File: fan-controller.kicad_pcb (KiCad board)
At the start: 2 copper layers, 33 x 16 mm, 17 parts, among them J1 PWR, J2 PTC, J3 FAN, J4 Prog, Q1 AO3401A, U1 PY32F002A

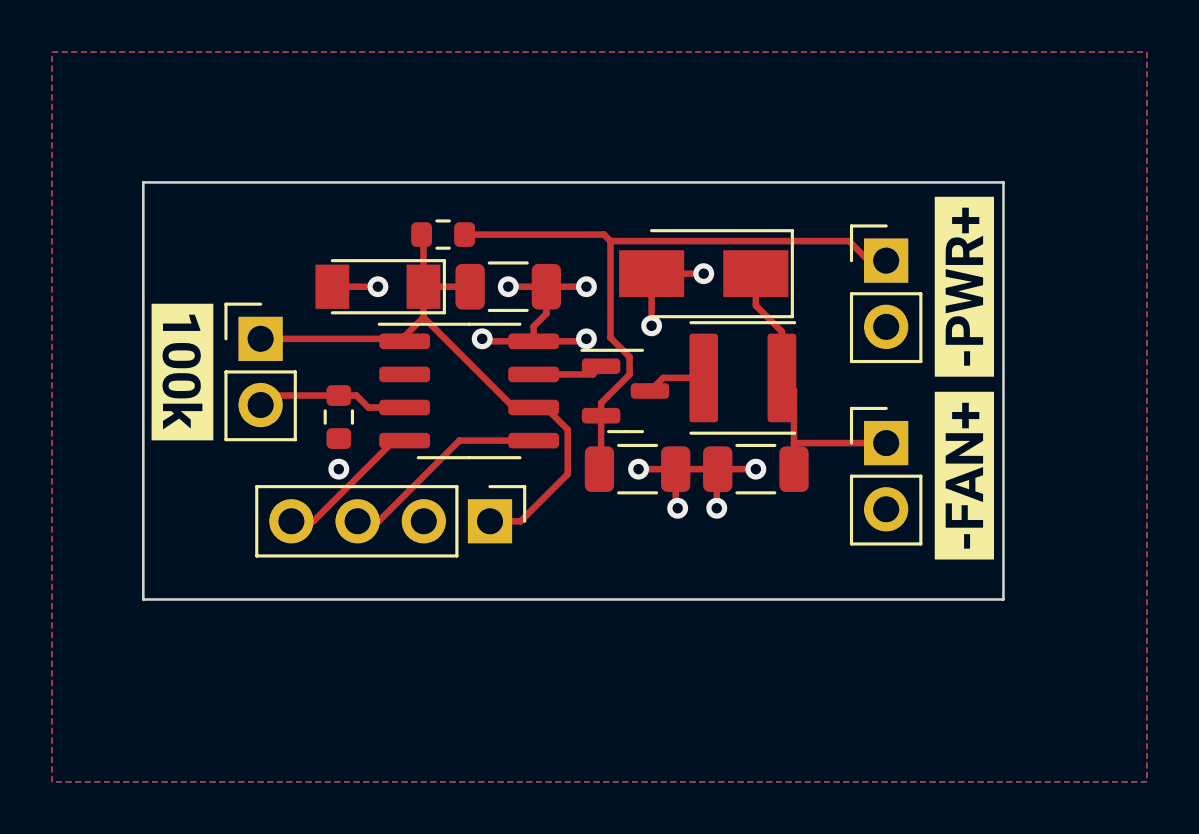
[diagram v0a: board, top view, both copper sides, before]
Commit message: Fix ERC
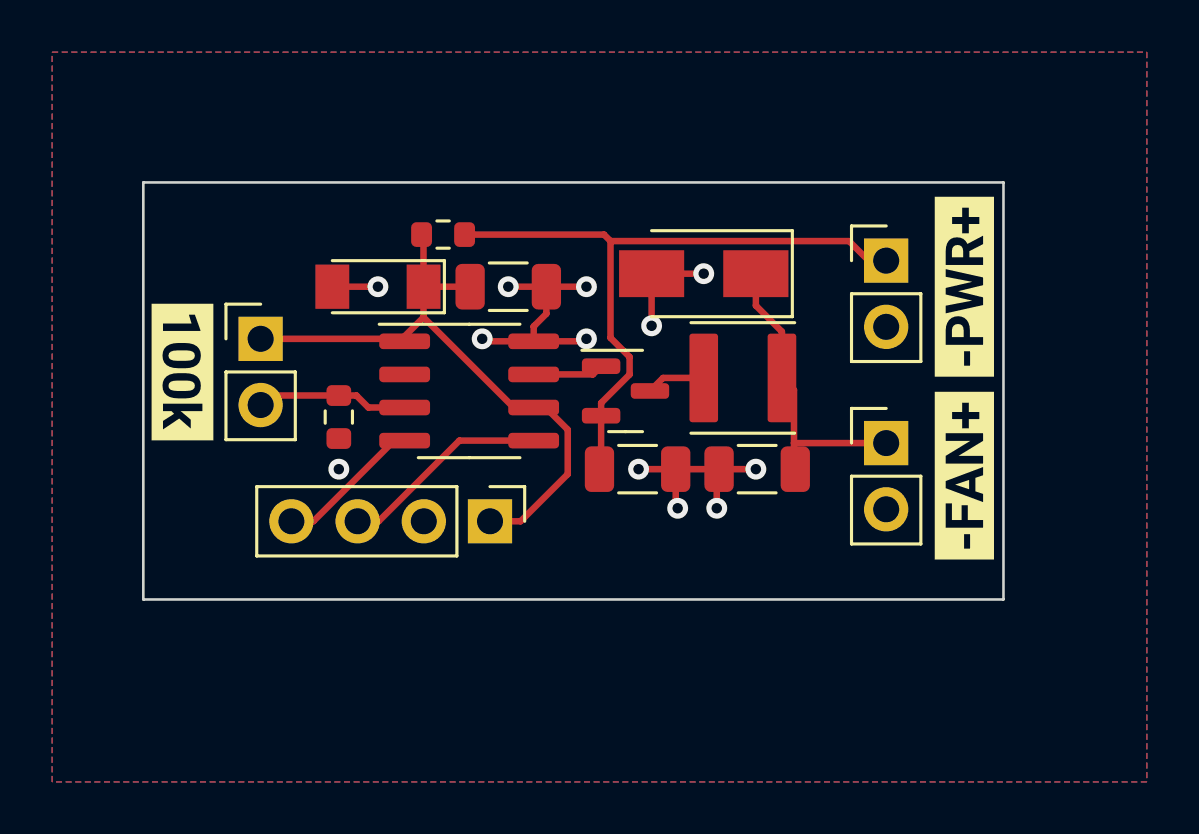
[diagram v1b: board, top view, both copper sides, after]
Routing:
- net +3.3V: track 24.8 -> 23.4 mm
- net VPP: track 26.6 -> 25.4 mm
- net Net-(C3-Pad1): track 12.1 -> 11.0 mm
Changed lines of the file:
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@@
     (tags "inductor abracon smd shielded")
     (property "LCSC" "C38117")
-    (property "Sheetfile" "/home/user/dev/hardware/fan-controller/fan-controller.sch")
+    (property "Sheetfile" "fan-controller.kicad_sch")
     (property "Sheetname" "")
     (attr smd)
@@
     (tags "resistor")
     (property "LCSC" "C25803")
-    (property "Sheetfile" "/home/user/dev/hardware/fan-controller/fan-controller.sch")
+    (property "Sheetfile" "fan-controller.kicad_sch")
     (property "Sheetname" "")
     (attr smd)
@@
     (property "Description" "50V+")
     (property "LCSC" "C13585")
-    (property "Sheetfile" "/home/user/dev/hardware/fan-controller/fan-controller.sch")
+    (property "Sheetfile" "fan-controller.kicad_sch")
     (property "Sheetname" "")
     (attr smd)
@@
   )
   (footprint "Resistor_SMD:R_1206_3216Metric" (layer "F.Cu")
-    (at 122 63 180)
+    (at 122.05 63 180)
     (descr "Resistor SMD 1206 (3216 Metric), square (rectangular) end terminal, IPC_7351 nominal, (Body size source: IPC-SM-782 page 72, https://www.pcb-3d.com/wordpress/wp-content/uploads/ipc-sm-782a_amendment_1_and_2.pdf), generated with kicad-footprint-generator")
     (tags "resistor")
     (property "Description" "50V+")
     (property "LCSC" "C13585")
-    (property "Sheetfile" "/home/user/dev/hardware/fan-controller/fan-controller.sch")
+    (property "Sheetfile" "fan-controller.kicad_sch")
     (property "Sheetname" "")
     (attr smd)
@@
     (descr "Through hole straight pin header, 1x02, 2.54mm pitch, single row")
     (tags "Through hole pin header THT 1x02 2.54mm single row")
-    (property "Sheetfile" "/home/user/dev/hardware/fan-controller/fan-controller.sch")
+    (property "Sheetfile" "fan-controller.kicad_sch")
     (property "Sheetname" "")
     (attr through_hole)
@@
     (descr "Through hole straight pin header, 1x02, 2.54mm pitch, single row")
     (tags "Through hole pin header THT 1x02 2.54mm single row")
-    (property "Sheetfile" "/home/user/dev/hardware/fan-controller/fan-controller.sch")
+    (property "Sheetfile" "fan-controller.kicad_sch")
     (property "Sheetname" "")
     (attr through_hole)
@@
     (tags "Diode Mini-MELF (SOD-80)")
     (property "LCSC" "C8056")
-    (property "Sheetfile" "/home/user/dev/hardware/fan-controller/fan-controller.sch")
+    (property "Sheetfile" "fan-controller.kicad_sch")
     (property "Sheetname" "")
     (attr smd)
@@
     (descr "Through hole straight pin header, 1x04, 2.54mm pitch, single row")
     (tags "Through hole pin header THT 1x04 2.54mm single row")
-    (property "Sheetfile" "/home/user/dev/hardware/fan-controller/fan-controller.sch")
+    (property "Sheetfile" "fan-controller.kicad_sch")
     (property "Sheetname" "")
     (attr through_hole)
@@
     (attr board_only exclude_from_pos_files exclude_from_bom)
     (fp_text reference "kibuzzard-63E17401" (at 0 -4.233917 90) (layer "F.SilkS") hide
-      (effects (font (size 0 0)))
+      (effects (font (size 0 0) (thickness 0.15)))
     )
     (fp_text value "G***" (at 0 4.233917 90) (layer "F.SilkS") hide
-      (effects (font (size 0 0)))
+      (effects (font (size 0 0) (thickness 0.15)))
     )
     (fp_poly (pts
@@
     (tags "resistor")
     (property "LCSC" "C25804")
-    (property "Sheetfile" "/home/user/dev/hardware/fan-controller/fan-controller.sch")
+    (property "Sheetfile" "fan-controller.kicad_sch")
     (property "Sheetname" "")
     (attr smd)
@@
     (attr board_only exclude_from_pos_files exclude_from_bom)
     (fp_text reference "kibuzzard-63E173EF" (at 0 -4.184695 90) (layer "F.SilkS") hide
-      (effects (font (size 0 0)))
+      (effects (font (size 0 0) (thickness 0.15)))
     )
     (fp_text value "G***" (at 0 4.184695 90) (layer "F.SilkS") hide
-      (effects (font (size 0 0)))
+      (effects (font (size 0 0) (thickness 0.15)))
     )
     (fp_poly (pts
@@
     (property "Description" "50V+")
     (property "LCSC" "C13585")
-    (property "Sheetfile" "/home/user/dev/hardware/fan-controller/fan-controller.sch")
+    (property "Sheetfile" "fan-controller.kicad_sch")
     (property "Sheetname" "")
     (attr smd)
@@
     (tags "Diode SMA (DO-214AC)")
     (property "LCSC" "C2480")
-    (property "Sheetfile" "/home/user/dev/hardware/fan-controller/fan-controller.sch")
+    (property "Sheetfile" "fan-controller.kicad_sch")
     (property "Sheetname" "")
     (attr smd)
@@
     (attr board_only exclude_from_pos_files exclude_from_bom)
     (fp_text reference "kibuzzard-63E173E4" (at 0 -4.184695 90) (layer "F.SilkS") hide
-      (effects (font (size 0 0)))
+      (effects (font (size 0 0) (thickness 0.15)))
     )
     (fp_text value "G***" (at 0 4.184695 90) (layer "F.SilkS") hide
-      (effects (font (size 0 0)))
+      (effects (font (size 0 0) (thickness 0.15)))
     )
     (fp_poly (pts
@@
     (tags "SOIC SO")
     (property "LCSC" "C5128435")
-    (property "Sheetfile" "/home/user/dev/hardware/fan-controller/fan-controller.sch")
+    (property "Sheetfile" "fan-controller.kicad_sch")
     (property "Sheetname" "")
     (attr smd)
@@
       (net 1 "+3.3V") (pinfunction "VCC") (pintype "power_in"))
     (pad "2" smd roundrect (at -2.475 -0.635) (size 1.95 0.6) (layers "F.Cu" "F.Paste" "F.Mask") (roundrect_rratio 0.25)
-      (net 10 "unconnected-(U1-Pad2)") (pinfunction "PA4/PA10") (pintype "bidirectional"))
+      (net 10 "unconnected-(U1-Pad2)") (pinfunction "PA4/PA10") (pintype "bidirectional+no_connect"))
     (pad "3" smd roundrect (at -2.475 0.635) (size 1.95 0.6) (layers "F.Cu" "F.Paste" "F.Mask") (roundrect_rratio 0.25)
       (net 5 "/TEMP_SENSE") (pinfunction "PA3") (pintype "bidirectional"))
@@
     (tags "SOT TO_SOT_SMD")
     (property "LCSC" "C15127")
-    (property "Sheetfile" "/home/user/dev/hardware/fan-controller/fan-controller.sch")
+    (property "Sheetfile" "fan-controller.kicad_sch")
     (property "Sheetname" "")
     (attr smd)
@@
     (descr "Through hole straight pin header, 1x02, 2.54mm pitch, single row")
     (tags "Through hole pin header THT 1x02 2.54mm single row")
-    (property "Sheetfile" "/home/user/dev/hardware/fan-controller/fan-controller.sch")
+    (property "Sheetfile" "fan-controller.kicad_sch")
     (property "Sheetname" "")
     (attr through_hole)
@@
   (segment (start 111.8 65) (end 112.9753 65) (width 0.25) (layer "F.Cu") (net 1))
   (segment (start 109.25 57.1753) (end 108.525 57.9003) (width 0.25) (layer "F.Cu") (net 1))
-  (segment (start 109.25 54.075) (end 109.175 54) (width 0.25) (layer "F.Cu") (net 1))
   (segment (start 111.0375 56) (end 109.25 56) (width 0.25) (layer "F.Cu") (net 1))
   (segment (start 109.25 56) (end 109.25 57.1753) (width 0.25) (layer "F.Cu") (net 1))
   (segment (start 112.9753 65) (end 114.783 63.1923) (width 0.25) (layer "F.Cu") (net 1))
-  (segment (start 112.7097 60.635) (end 113.475 60.635) (width 0.25) (layer "F.Cu") (net 1))
   (segment (start 109.25 57.1753) (end 112.7097 60.635) (width 0.25) (layer "F.Cu") (net 1))
-  (segment (start 113.933 60.635) (end 113.475 60.635) (width 0.25) (layer "F.Cu") (net 1))
-  (segment (start 108.525 58) (end 108.525 58.095) (width 0.25) (layer "F.Cu") (net 1))
   (segment (start 108.525 57.9003) (end 108.525 58) (width 0.25) (layer "F.Cu") (net 1))
   (segment (start 114.783 63.1923) (end 114.783 61.485) (width 0.25) (layer "F.Cu") (net 1))
@@
   (segment (start 122 63) (end 121 63) (width 0.25) (layer "F.Cu") (net 2))
   (segment (start 113.9625 56) (end 113.9625 57.0375) (width 0.25) (layer "F.Cu") (net 2))
-  (segment (start 113.9625 56) (end 114 56.0375) (width 0.25) (layer "F.Cu") (net 2))
   (segment (start 115.405 58.095) (end 115.5 58) (width 0.25) (layer "F.Cu") (net 2))
   (segment (start 113.475 58.095) (end 111.595 58.095) (width 0.25) (layer "F.Cu") (net 2))
@@
   (segment (start 116.0625 60.95) (end 116.0625 60.4625) (width 0.25) (layer "F.Cu") (net 3))
   (segment (start 116.4246 57.9644) (end 116.4246 54.25) (width 0.25) (layer "F.Cu") (net 3))
-  (segment (start 116 63) (end 116.0625 62.9375) (width 0.25) (layer "F.Cu") (net 3))
-  (segment (start 127.5 55) (end 126.3247 55) (width 0.25) (layer "F.Cu") (net 3))
   (segment (start 116.0625 62.9375) (end 116.0625 60.95) (width 0.25) (layer "F.Cu") (net 3))
   (segment (start 123 57.7253) (end 122 56.7253) (width 0.25) (layer "F.Cu") (net 4))
-  (segment (start 127.5 62) (end 126.3247 62) (width 0.25) (layer "F.Cu") (net 4))
   (segment (start 123.4625 59.9625) (end 123 59.5) (width 0.25) (layer "F.Cu") (net 4))
   (segment (start 123 59.5) (end 123 57.7253) (width 0.25) (layer "F.Cu") (net 4))
@@
   (segment (start 123.4625 62) (end 126.3247 62) (width 0.25) (layer "F.Cu") (net 4))
   (segment (start 122 55.5) (end 122 56.7253) (width 0.25) (layer "F.Cu") (net 4))
-  (segment (start 106 60.3575) (end 106 60.175) (width 0.25) (layer "F.Cu") (net 5))
   (segment (start 106 60.175) (end 102.825 60.175) (width 0.25) (layer "F.Cu") (net 5))
   (segment (start 108.525 60.635) (end 107.135 60.635) (width 0.25) (layer "F.Cu") (net 5))
@@
   (segment (start 110.6229 61.905) (end 113.475 61.905) (width 0.25) (layer "F.Cu") (net 6))
   (segment (start 107.5279 65) (end 110.6229 61.905) (width 0.25) (layer "F.Cu") (net 6))
-  (segment (start 108.1209 61.905) (end 108.525 61.905) (width 0.25) (layer "F.Cu") (net 7))
   (segment (start 105.0259 65) (end 108.1209 61.905) (width 0.25) (layer "F.Cu") (net 7))
   (segment (start 104.18 65) (end 105.0259 65) (width 0.25) (layer "F.Cu") (net 7))
